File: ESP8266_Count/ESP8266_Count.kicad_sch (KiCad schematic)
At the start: 26 parts, among them J1 PMG, J2 String1, J3 OLED, SW1 SW_Push, U1 AMS1117-3.3, U2 AMS1117-5.0, U3 ESP-12E, U4 74AHCT1G125, U5 ACS706xLC-05C

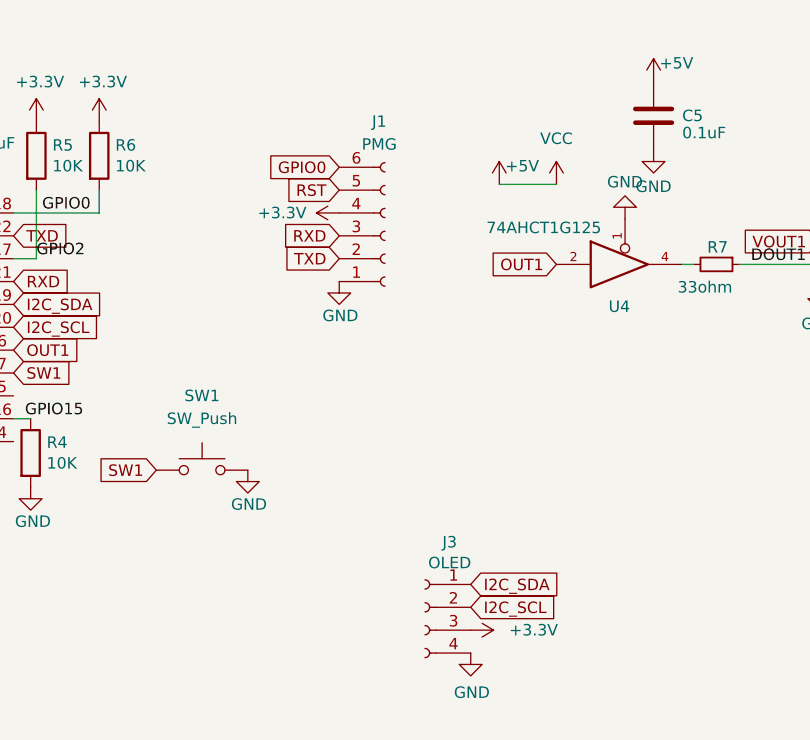
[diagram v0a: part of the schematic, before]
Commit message: minor fixes
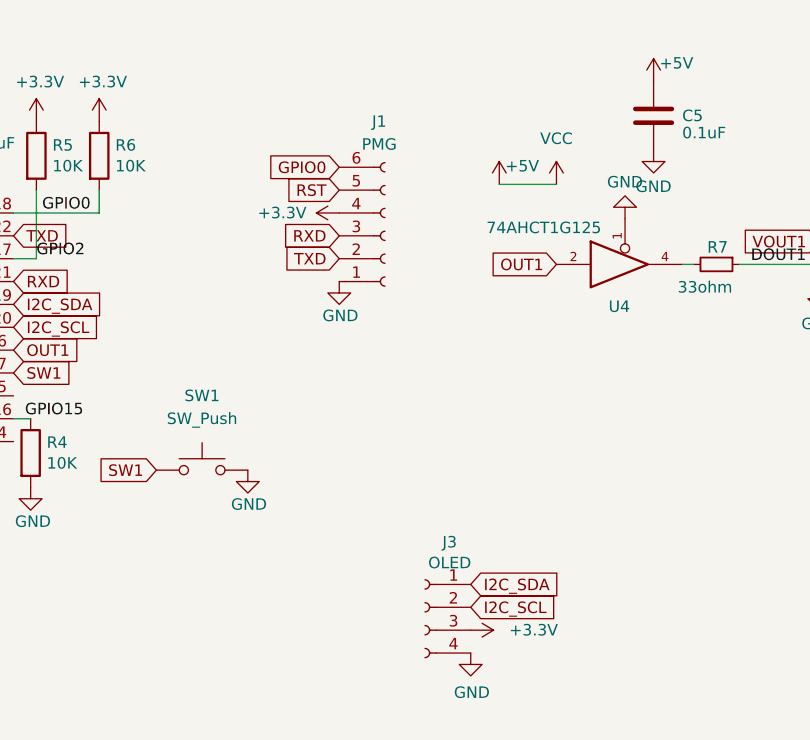
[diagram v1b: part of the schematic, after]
